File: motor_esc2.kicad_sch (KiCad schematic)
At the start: 14 parts, among them J5 SolderWirePad_1x01_SMD_3x6mm, J6 SolderWirePad_1x01_SMD_3x6mm, J7 SolderWirePad_1x01_SMD_3x6mm, U5 MCF8316A

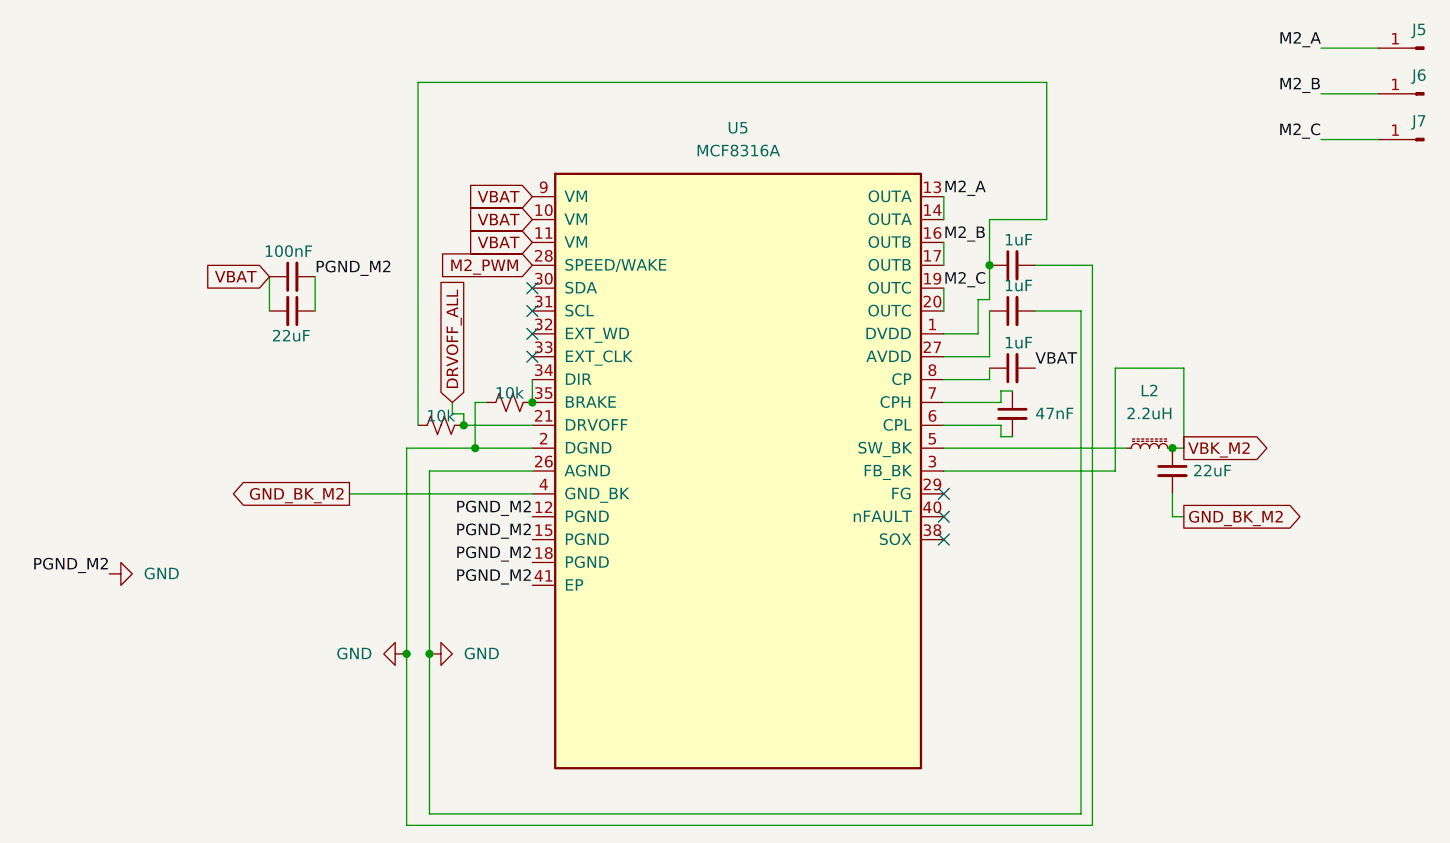
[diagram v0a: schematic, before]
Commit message: done?
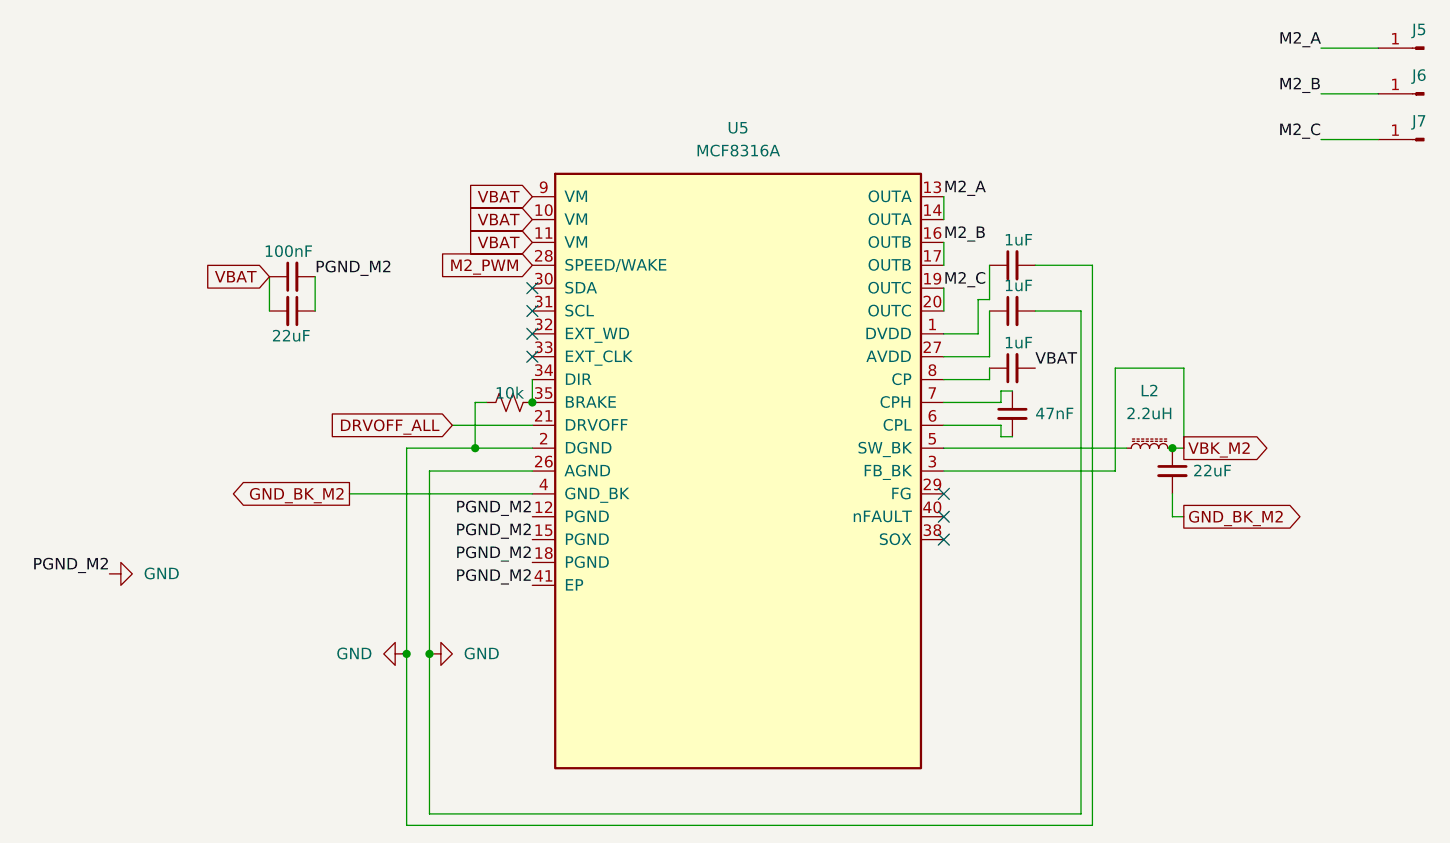
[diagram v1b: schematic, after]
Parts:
- removed R7: 10k, Resistor_SMD:R_0603_1608Metric_Pad0.98x0.95mm_HandSolder, symbol Device:R_Small_US
- R9: footprint Resistor_SMD:R_0603_1608Metric_Pad0.98x0.95mm_HandSolder -> Resistor_SMD:R_0402_1005Metric_Pad0.72x0.64mm_HandSolder
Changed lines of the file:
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@@
-	)
-	(junction
-		(at 160.02 62.23)
-		(diameter 0)
-		(color 0 0 0 0)
 	)
 	(junction
@@
 	)
 	(junction
-		(at 101.6 80.01)
-		(diameter 0)
-		(color 0 0 0 0)
-	)
-	(junction
 		(at 102.87 82.55)
 		(diameter 0)
@@
 	(wire
 		(pts
+			(xy 100.33 80.01) (xy 109.22 80.01)
+		)
+		(stroke
+			(width 0)
+			(type default)
+		)
+	)
+	(wire
+		(pts
 			(xy 158.75 69.85) (xy 158.75 66.04)
 		)
@@
 	(wire
 		(pts
-			(xy 166.37 41.91) (xy 166.37 57.15)
-		)
-		(stroke
-			(width 0)
-			(type default)
-		)
-	)
-	(wire
-		(pts
 			(xy 80.01 63.5) (xy 80.01 67.31)
 		)
@@
 	(wire
 		(pts
-			(xy 166.37 41.91) (xy 96.52 41.91)
-		)
-		(stroke
-			(width 0)
-			(type default)
-		)
-	)
-	(wire
-		(pts
 			(xy 171.45 124.46) (xy 95.25 124.46)
 		)
@@
 	(wire
 		(pts
-			(xy 100.33 78.74) (xy 101.6 78.74)
-		)
-		(stroke
-			(width 0)
-			(type default)
-		)
-	)
-	(wire
-		(pts
 			(xy 161.29 80.01) (xy 154.94 80.01)
 		)
@@
 	(wire
 		(pts
-			(xy 166.37 57.15) (xy 160.02 57.15)
-		)
-		(stroke
-			(width 0)
-			(type default)
-		)
-	)
-	(wire
-		(pts
 			(xy 170.18 123.19) (xy 97.79 123.19)
 		)
@@
 	(wire
 		(pts
-			(xy 100.33 77.47) (xy 100.33 78.74)
-		)
-		(stroke
-			(width 0)
-			(type default)
-		)
-	)
-	(wire
-		(pts
-			(xy 96.52 41.91) (xy 96.52 80.01)
-		)
-		(stroke
-			(width 0)
-			(type default)
-		)
-	)
-	(wire
-		(pts
 			(xy 154.94 64.77) (xy 154.94 67.31)
 		)
@@
 	(wire
 		(pts
-			(xy 101.6 78.74) (xy 101.6 80.01)
-		)
-		(stroke
-			(width 0)
-			(type default)
-		)
-	)
-	(wire
-		(pts
 			(xy 203.2 48.26) (xy 196.85 48.26)
 		)
@@
 	(wire
 		(pts
-			(xy 160.02 57.15) (xy 160.02 62.23)
-		)
-		(stroke
-			(width 0)
-			(type default)
-		)
-	)
-	(wire
-		(pts
 			(xy 154.94 85.09) (xy 173.99 85.09)
 		)
@@
 		(pts
 			(xy 109.22 74.93) (xy 109.22 77.47)
-		)
-		(stroke
-			(width 0)
-			(type default)
-		)
-	)
-	(wire
-		(pts
-			(xy 101.6 80.01) (xy 109.22 80.01)
 		)
 		(stroke
@@
 	(global_label "DRVOFF_ALL"
 		(shape input)
-		(at 100.33 77.47 90)
+		(at 100.33 80.01 180)
 		(fields_autoplaced yes)
 		(effects
@@
 				(size 1.27 1.27)
 			)
-			(justify left)
+			(justify right)
 		)
 		(property "Intersheetrefs" "${INTERSHEET_REFS}"
-			(at 100.33 63.2361 90)
-			(effects
-				(font
-					(size 1.27 1.27)
-				)
-				(justify left)
+			(at 86.0961 80.01 0)
+			(effects
+				(font
+					(size 1.27 1.27)
+				)
+				(justify right)
 				(hide yes)
 			)
@@
 				(path "/ec430d83-72cd-4950-a197-fb5338d7c552/095f9007-0d78-4904-a8f3-9d4f0ede6e86"
 					(reference "C27")
-					(unit 1)
-				)
-			)
-		)
-	)
-	(symbol
-		(lib_id "Device:R_Small_US")
-		(at 99.06 80.01 90)
-		(unit 1)
-		(exclude_from_sim no)
-		(in_bom yes)
-		(on_board yes)
-		(dnp no)
-		(property "Reference" "R7"
-			(at 99.06 73.66 90)
-			(effects
-				(font
-					(size 1.27 1.27)
-				)
-				(hide yes)
-			)
-		)
-		(property "Value" "10k"
-			(at 99.06 78.994 90)
-			(effects
-				(font
-					(size 1.27 1.27)
-				)
-			)
-		)
-		(property "Footprint" "Resistor_SMD:R_0603_1608Metric_Pad0.98x0.95mm_HandSolder"
-			(at 99.06 80.01 0)
-			(effects
-				(font
-					(size 1.27 1.27)
-				)
-				(hide yes)
-			)
-		)
-		(property "Datasheet" "~"
-			(at 99.06 80.01 0)
-			(effects
-				(font
-					(size 1.27 1.27)
-				)
-				(hide yes)
-			)
-		)
-		(property "Description" "Resistor, small US symbol"
-			(at 99.06 80.01 0)
-			(effects
-				(font
-					(size 1.27 1.27)
-				)
-				(hide yes)
-			)
-		)
-		(pin "2"
-		)
-		(pin "1"
-		)
-		(instances
-			(project "neodrone-v1"
-				(path "/ec430d83-72cd-4950-a197-fb5338d7c552/095f9007-0d78-4904-a8f3-9d4f0ede6e86"
-					(reference "R7")
 					(unit 1)
 				)
@@
 			)
 		)
-		(property "Footprint" "Resistor_SMD:R_0603_1608Metric_Pad0.98x0.95mm_HandSolder"
+		(property "Footprint" "Resistor_SMD:R_0402_1005Metric_Pad0.72x0.64mm_HandSolder"
 			(at 106.68 77.47 0)
 			(effects
@@
 			)
 		)
-		(property "Datasheet" "~"
+		(property "Datasheet" ""
 			(at 106.68 77.47 0)
 			(effects
@@
 			)
 		)
-		(property "Description" "Resistor, small US symbol"
+		(property "Description" ""
 			(at 106.68 77.47 0)
 			(effects
